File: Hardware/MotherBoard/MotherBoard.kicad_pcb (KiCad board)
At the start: 2 copper layers, 145 x 160 mm, 45 parts, among them J1 POWER, J10 I/O_PWR, J2 I/O0, J3 ISA00, J4 ISA10, J5 I/O1, J6 EXTRN_CLCK, J7 ISA01, J8 ISA11, J9 Conn_02x02_Odd_Even, SW1 SW_Push, U1 AMS1117-5.0, U10 74HCT541, U11 SN74LVC245AN, U12 SN74LVC245AN, U13 74HCT541, U14 74HCT541, U2 28C256, U3 WD65C22, U4 HM62256BLP, U5 WD65C02, U6 4012, U7 4023, U8 4069, U9 74HCT541, X1 ACO-1MHz

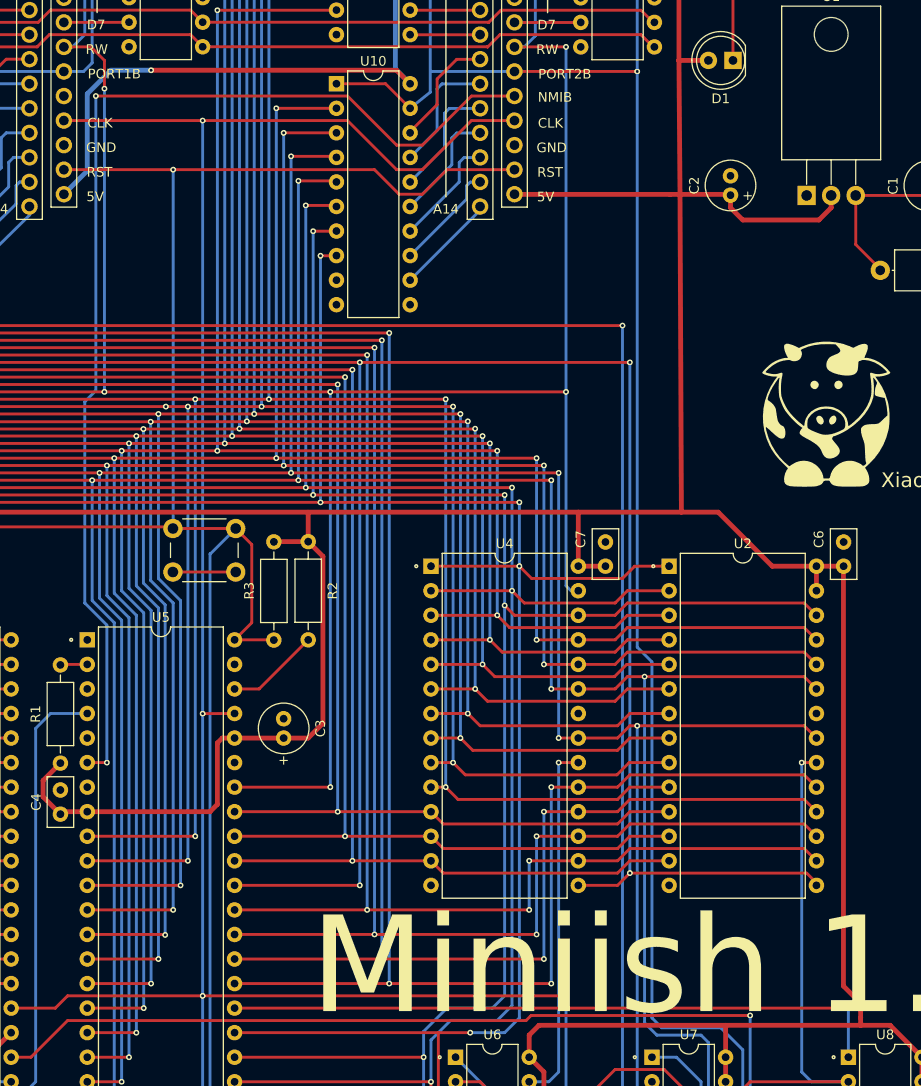
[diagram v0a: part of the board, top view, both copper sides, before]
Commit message: Fix
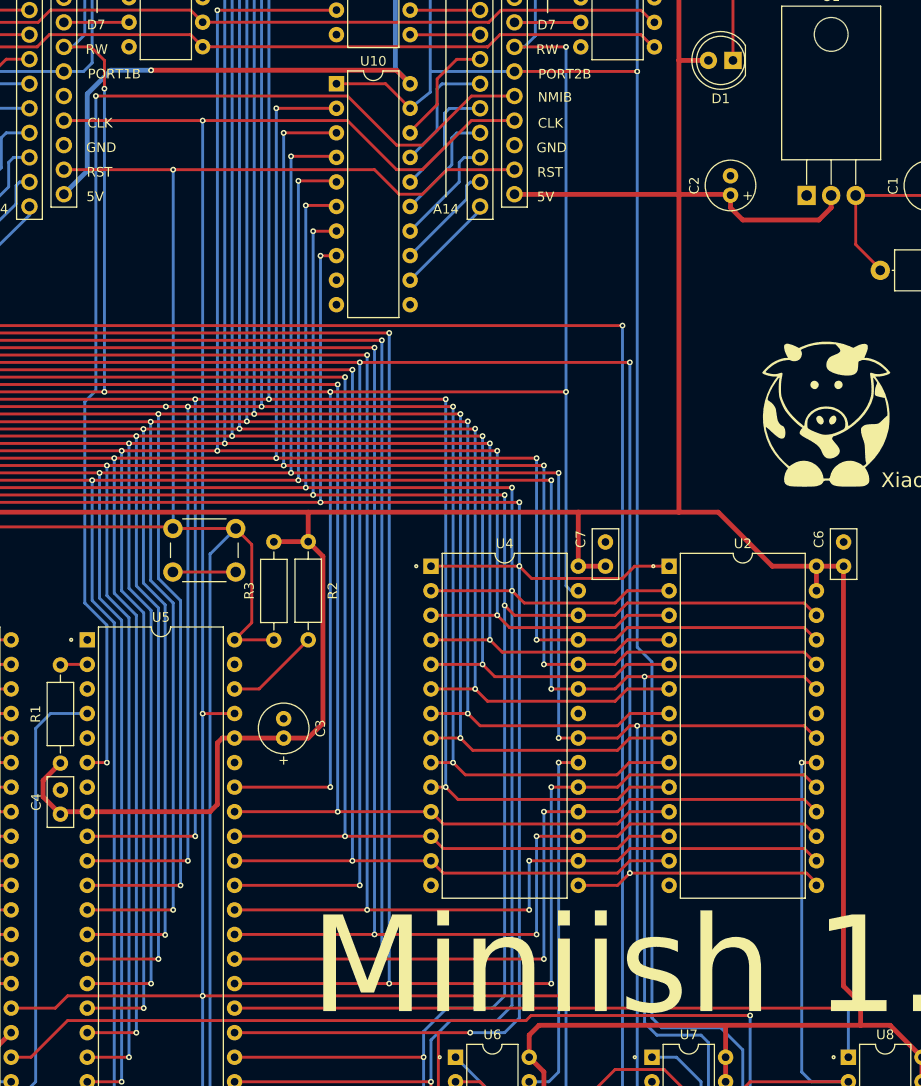
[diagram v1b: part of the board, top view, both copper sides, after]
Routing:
- net +5V: track 751.4 -> 750.5 mm
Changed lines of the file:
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@@
   (segment (start 145.542 68.3255) (end 145.542 73.4055) (width 0.3) (layer "F.Cu") (net 2))
   (segment (start 98.044 55.372) (end 99.441 56.769) (width 0.5) (layer "F.Cu") (net 3))
-  (segment (start 127.2545 54.3555) (end 127.254 54.356) (width 0.5) (layer "F.Cu") (net 3))
   (segment (start 77.979853 30.083285) (end 81.012138 27.051) (width 0.5) (layer "F.Cu") (net 3))
   (segment (start 63.263 127.055831) (end 61.468 128.850831) (width 0.5) (layer "F.Cu") (net 3))
   (segment (start 52.74152 28.973999) (end 53.140519 28.575) (width 0.5) (layer "F.Cu") (net 3))
   (segment (start 50.545 162.56) (end 58.165 154.94) (width 0.5) (layer "F.Cu") (net 3))
+  (segment (start 127.2545 54.3555) (end 127.254 68.326) (width 0.5) (layer "F.Cu") (net 3))
   (segment (start 66.04 132.08) (end 78.74 132.08) (width 0.5) (layer "F.Cu") (net 3))
   (segment (start 81.28 124.46) (end 86.36 124.46) (width 0.5) (layer "F.Cu") (net 3))
   (segment (start 86.36 124.46) (end 88.9 124.46) (width 0.5) (layer "F.Cu") (net 3))
   (segment (start 81.28 124.46) (end 80.01 124.46) (width 0.5) (layer "F.Cu") (net 3))
-  (segment (start 146.05 153.416) (end 146.05 154.178) (width 0.5) (layer "F.Cu") (net 3))
+  (segment (start 146.05 151.892) (end 146.05 154.178) (width 0.5) (layer "F.Cu") (net 3))
   (segment (start 80.01 124.46) (end 79.502 124.968) (width 0.5) (layer "F.Cu") (net 3))
   (segment (start 152.4 160.02) (end 152.4 157.48) (width 0.5) (layer "F.Cu") (net 3))
   (segment (start 133.8575 70.8655) (end 141.733 70.8655) (width 0.5) (layer "F.Cu") (net 3))
+  (segment (start 127.254 68.326) (end 127.254 101.092) (width 0.5) (layer "F.Cu") (net 3))
+  (segment (start 116.84 101.092) (end 127.254 101.092) (width 0.5) (layer "F.Cu") (net 3))
   (segment (start 88.9 101.092) (end 88.9 104.14) (width 0.5) (layer "F.Cu") (net 3))
   (segment (start 111.76 157.48) (end 111.76 155.194) (width 0.5) (layer "F.Cu") (net 3))
@@
   (segment (start 50.546 162.56) (end 58.42 170.763903) (width 0.5) (layer "F.Cu") (net 3))
   (segment (start 155.194 179.832) (end 153.416 181.61) (width 0.5) (layer "F.Cu") (net 3))
-  (segment (start 126.363147 68.214715) (end 110.226918 68.214715) (width 0.5) (layer "F.Cu") (net 3))
   (segment (start 116.84 106.68) (end 116.84 101.092) (width 0.5) (layer "F.Cu") (net 3))
   (segment (start 116.84 106.68) (end 119.651 106.68) (width 0.5) (layer "F.Cu") (net 3))
@@
   (segment (start 123.078715 28.590715) (end 124.714 30.099) (width 0.5) (layer "F.Cu") (net 3))
   (segment (start 131.318 101.092) (end 136.906 106.68) (width 0.5) (layer "F.Cu") (net 3))
-  (segment (start 63.263 132.334) (end 63.517 132.08) (width 0.5) (layer "F.Cu") (net 3))
   (segment (start 149.098 154.178) (end 146.05 154.178) (width 0.5) (layer "F.Cu") (net 3))
+  (segment (start 127.363432 68.216568) (end 132.510578 68.216568) (width 0.5) (layer "F.Cu") (net 3))
   (segment (start 127.254 54.355) (end 127.254 32.639) (width 0.5) (layer "F.Cu") (net 3))
   (segment (start 81.026 181.61) (end 78.74 179.324) (width 0.5) (layer "F.Cu") (net 3))
   (segment (start 40.148 162.56) (end 42.925 162.56) (width 0.5) (layer "F.Cu") (net 3))
   (segment (start 90.424 122.936) (end 90.424 105.664) (width 0.5) (layer "F.Cu") (net 3))
+  (segment (start 127.254 101.092) (end 131.318 101.092) (width 0.5) (layer "F.Cu") (net 3))
   (segment (start 81.012138 27.051) (end 97.663 27.051) (width 0.5) (layer "F.Cu") (net 3))
   (segment (start 130.302 54.3555) (end 127.2545 54.3555) (width 0.5) (layer "F.Cu") (net 3))
@@
   (segment (start 153.416 181.61) (end 81.026 181.61) (width 0.5) (layer "F.Cu") (net 3))
   (segment (start 79.502 131.318) (end 78.74 132.08) (width 0.5) (layer "F.Cu") (net 3))
-  (segment (start 126.365 68.216568) (end 132.510578 68.216568) (width 0.5) (layer "F.Cu") (net 3))
   (segment (start 63.517 132.08) (end 65.532 132.08) (width 0.5) (layer "F.Cu") (net 3))
-  (segment (start 126.363147 68.214715) (end 126.365 68.216568) (width 0.5) (layer "F.Cu") (net 3))
   (segment (start 141.478 106.68) (end 144.289 106.68) (width 0.5) (layer "F.Cu") (net 3))
   (segment (start 99.747666 28.590715) (end 123.078715 28.590715) (width 0.5) (layer "F.Cu") (net 3))
@@
   (segment (start 61.468 130.539) (end 63.263 132.334) (width 0.5) (layer "F.Cu") (net 3))
   (segment (start 127.2545 54.3555) (end 127.254 54.355) (width 0.5) (layer "F.Cu") (net 3))
-  (segment (start 65.532 132.08) (end 66.04 132.08) (width 0.5) (layer "F.Cu") (net 3))
   (segment (start 111.76 155.194) (end 112.776 154.178) (width 0.5) (layer "F.Cu") (net 3))
   (segment (start 61.468 128.850831) (end 61.468 130.539) (width 0.5) (layer "F.Cu") (net 3))
@@
   (segment (start 132.08 157.48) (end 132.08 160.02) (width 0.5) (layer "F.Cu") (net 3))
   (segment (start 132.588 68.29399) (end 132.588 69.596) (width 0.5) (layer "F.Cu") (net 3))
+  (segment (start 110.226918 68.214715) (end 127.363432 68.216568) (width 0.5) (layer "F.Cu") (net 3))
   (segment (start 76.471568 28.575) (end 77.979853 30.083285) (width 0.5) (layer "F.Cu") (net 3))
   (segment (start 58.42 170.763903) (end 70.358 170.763903) (width 0.5) (layer "F.Cu") (net 3))
   (segment (start 97.663 27.051) (end 99.441 28.829) (width 0.5) (layer "F.Cu") (net 3))
-  (segment (start 127.254 54.356) (end 127.363432 68.216568) (width 0.5) (layer "F.Cu") (net 3))
   (segment (start 111.76 157.48) (end 113.284 159.004) (width 0.5) (layer "F.Cu") (net 3))
   (segment (start 70.358 170.763903) (end 78.74 179.324) (width 0.5) (layer "F.Cu") (net 3))
-  (segment (start 127.363432 68.216568) (end 127.508 101.092) (width 0.5) (layer "F.Cu") (net 3))
-  (segment (start 146.05 151.892) (end 146.05 153.416) (width 0.5) (layer "F.Cu") (net 3))
   (segment (start 127.254 32.639) (end 124.714 30.099) (width 0.5) (layer "F.Cu") (net 3))
-  (segment (start 116.84 101.092) (end 131.318 101.092) (width 0.5) (layer "F.Cu") (net 3))
   (segment (start 90.424 105.664) (end 88.9 104.14) (width 0.5) (layer "F.Cu") (net 3))
-  (segment (start 144.289 106.68) (end 144.272 106.697) (width 0.5) (layer "F.Cu") (net 3))
   (segment (start 72.644 55.372) (end 98.044 55.372) (width 0.5) (layer "F.Cu") (net 3))
   (segment (start 136.906 106.68) (end 141.478 106.68) (width 0.5) (layer "F.Cu") (net 3))
